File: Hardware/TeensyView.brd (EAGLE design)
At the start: 160 x 100 mm, 9 parts

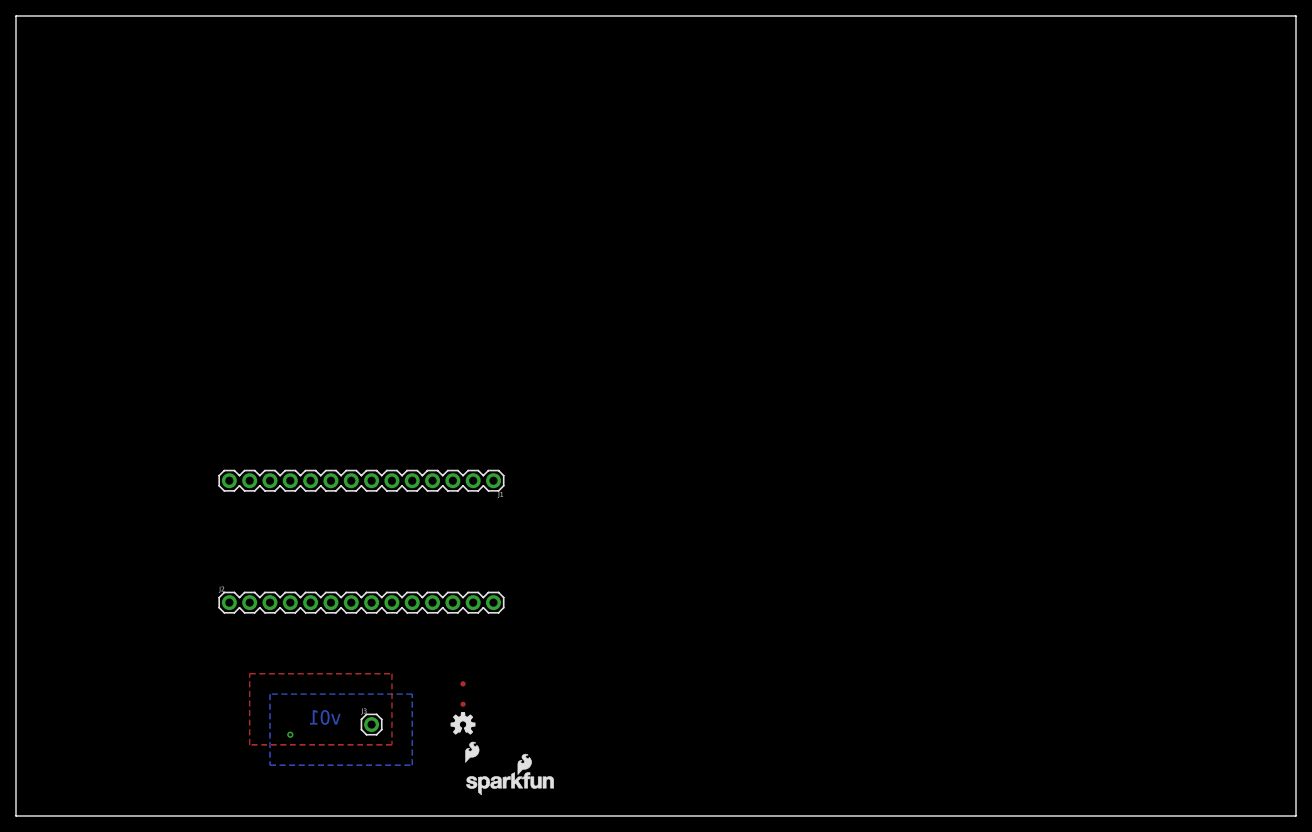
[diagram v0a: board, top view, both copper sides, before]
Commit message: Proto 1 design complete
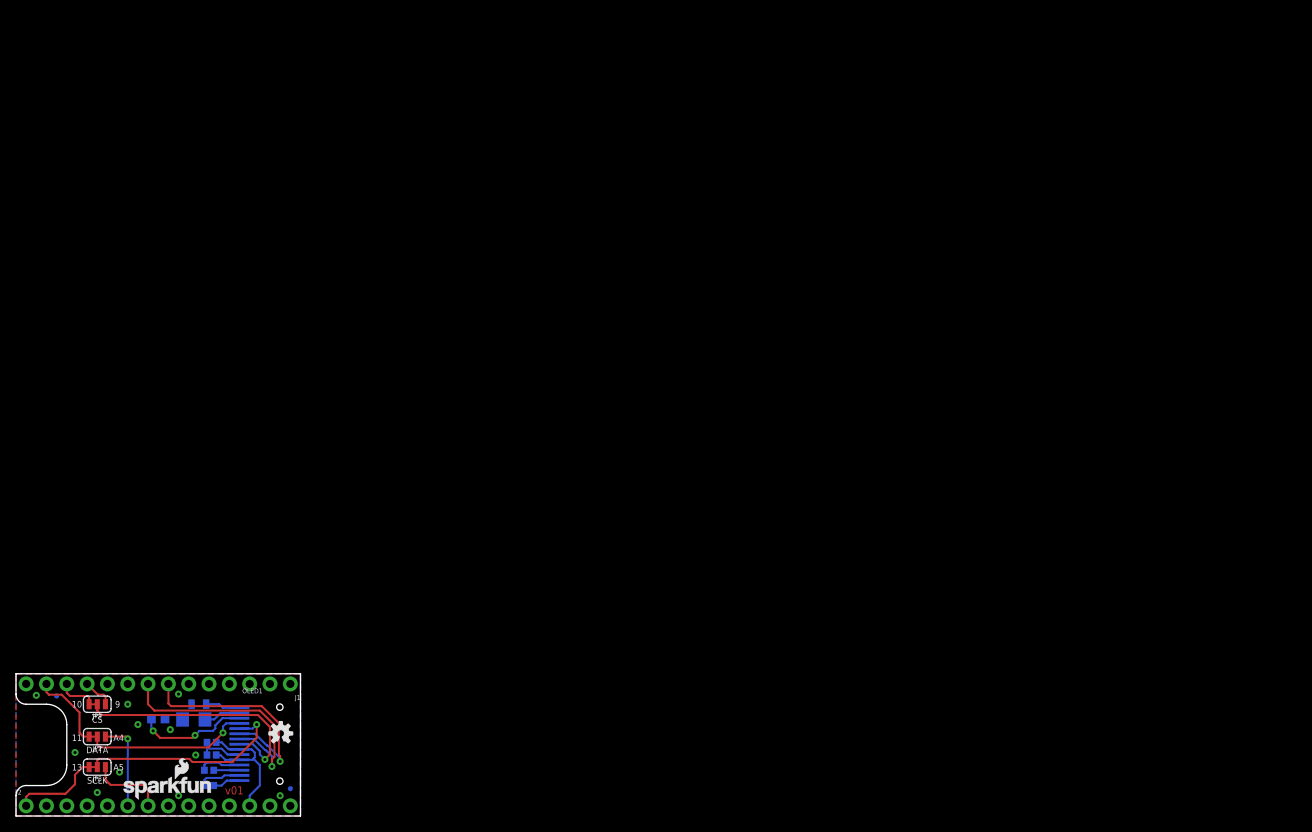
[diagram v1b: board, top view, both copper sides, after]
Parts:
- removed J3: (no value), SparkFun-Connectors:1X01
- added C1, C2, C3, C4: 1.0uF, SparkFun-Capacitors:0402
- added C5: 2.2uF, SparkFun-Capacitors:0805
- added C6: 4.7UF, SparkFun-Capacitors:1206
- added JP1, JP2, JP3: JUMPER-SMT_3_1-NC_TRACE_SILK, SparkFun-Jumpers:SMT-JUMPER_3_1-NC_TRACE_SILK
- added OLED1: OLED128X64SIDEREAR-MOUNT, TeensyViewDev:OLED-UG-2832TSWGG01-REAR
- added R1: 330k, SparkFun-Resistors:0603
- J1, J2: value (none) -> DNP; device SparkFun-Connectors:1X14 -> SparkFun-Connectors:1X14_NO_SILK
- moved FD2 50.8 mm to (5.08, 15.0), flipped to the bottom
- moved LOGO1 46.2 mm to (9.92, 11.0), flipped to the bottom
- moved LOGO3 42.9 mm to (13.0, 1.98)
- moved J2 35.9 mm to (1.27, 1.27)
- moved J1 35.9 mm to (34.3, 16.5)
- moved FD1 25.3 mm to (34.3, 3.41), flipped to the bottom
- moved LOGO2 22.8 mm to (33.1, 10.3)
- moved FRAME1 16.3 mm to (-14.0, -24.1)
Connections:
- new net !CS: JP1.2, OLED1.8
- new net !RESET: J1.8, OLED1.9
- new net D/!C: J1.7, OLED1.10
- new net N$1: J1.12, JP1.3
- new net N$10: J2.1, JP3.3
- new net N$11: J2.7, JP3.1
- new net N$12: J1.13, JP2.3
- new net N$13: J2.6, JP2.1
- new net N$2: J1.11, JP1.1
- new net N$3: C4.2, OLED1.4
- new net N$4: C4.1, OLED1.3
- new net N$5: C3.2, OLED1.2
- new net N$6: C3.1, OLED1.1
- new net N$7: OLED1.13, R1.2
- new net N$8: C6.1, OLED1.14
- new net N$9: C5.1, OLED1.15
- new net SCLK: JP3.2, OLED1.11
- new net SDIN: JP2.2, OLED1.12
- new net VCC: C1.1, C2.1, J2.12, OLED1.5, OLED1.7
- net GND: now also C1.2, C2.2, C5.2, C6.2, J1.1, OLED1.6, R1.1; no longer J3.1
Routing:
- net !CS: track 0.00 -> 31.8 mm, vias 0 -> 1
- net !RESET: track 0.00 -> 30.9 mm, vias 0 -> 1
- net D/!C: track 0.00 -> 28.9 mm, vias 0 -> 1
- net SCLK: track 0.00 -> 26.3 mm, vias 0 -> 1
- net SDIN: track 0.00 -> 20.6 mm, vias 0 -> 1
- net VCC: track 0.00 -> 17.9 mm
- net N$7: track 0.00 -> 13.9 mm, vias 0 -> 2
- net N$13: track 0.00 -> 11.3 mm, vias 0 -> 1
- net N$10: track 0.00 -> 11.2 mm
- net N$12: track 0.00 -> 10.2 mm
- net N$11: track 0.00 -> 9.47 mm
- net GND: track 0.00 -> 5.95 mm, vias 1 -> 11
- net N$3: track 0.00 -> 5.32 mm
- net N$5: track 0.00 -> 5.31 mm
- net N$1: track 0.00 -> 5.00 mm
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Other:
- board size 160 x 100 mm -> 35.6 x 17.8 mm
- board text added: "!CS"
- board text added: "10"
- board text added: "11"
- board text added: "13"
- board text added: "9"
- board text added: "A4"
- board text added: "A5"
- board text added: "DATA"
- board text added: "Measurements in inches"
- board text added: "SCLK"
- board text added: "TeensyView"
